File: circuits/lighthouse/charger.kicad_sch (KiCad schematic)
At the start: 15 parts, among them Q2 FS8205A, U4 TP4056-42-ESOP8, U5 DW01A

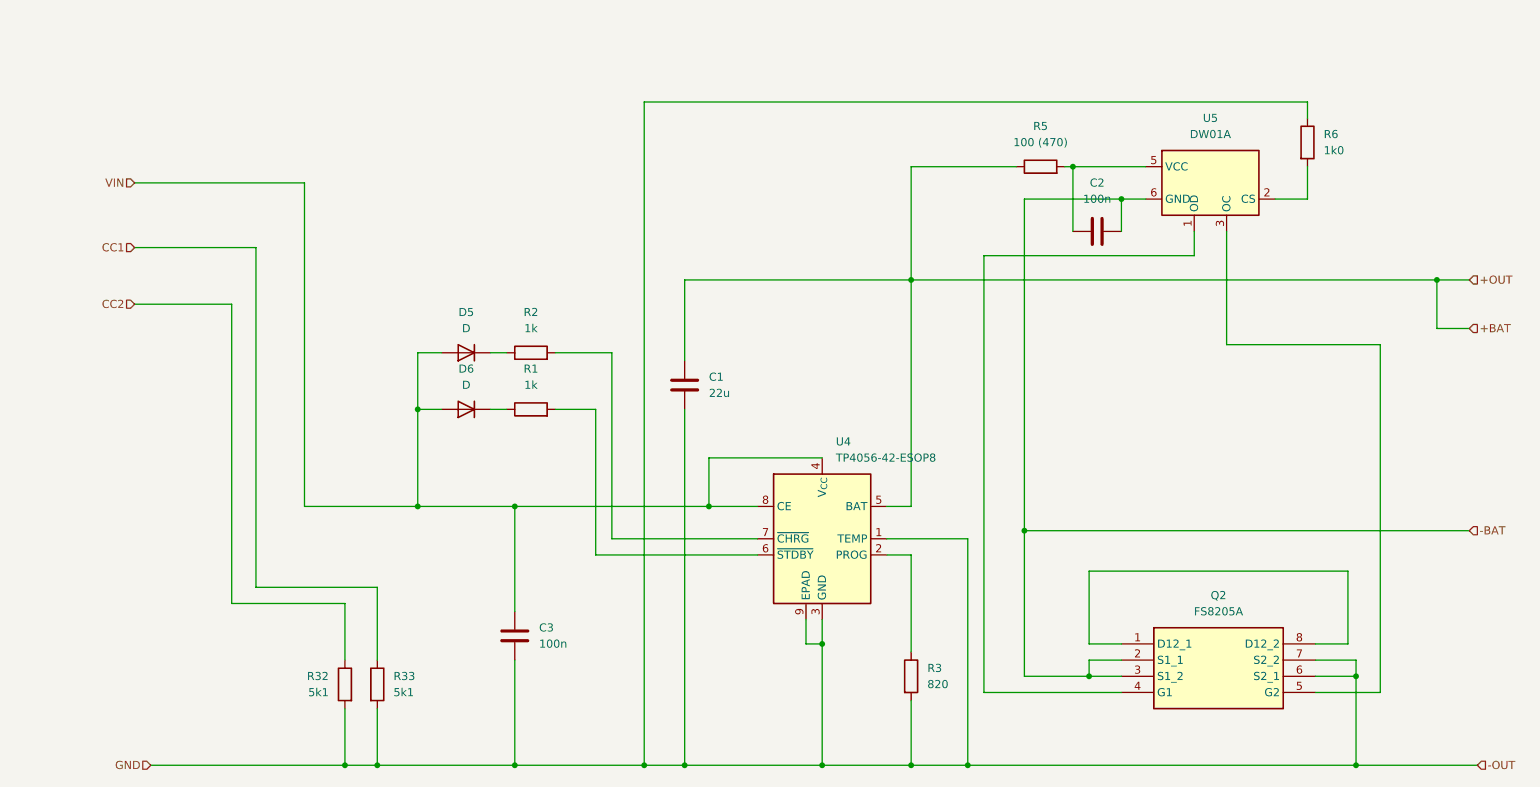
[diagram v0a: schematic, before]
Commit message: Cleaned up schematics
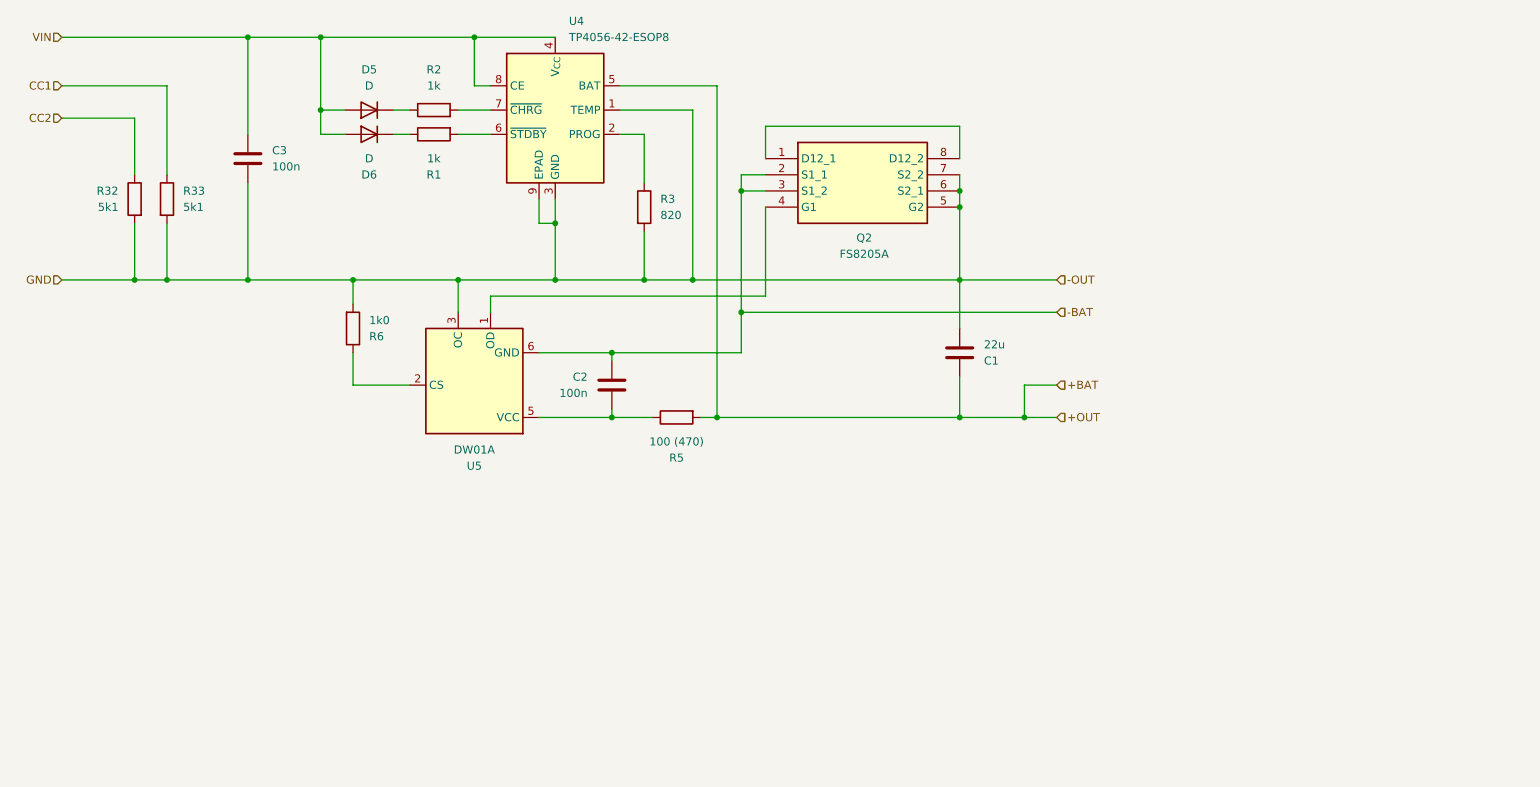
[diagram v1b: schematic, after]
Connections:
- net +BAT: now also R5.2; no longer R5.1
- net -OUT: now also Q2.5 (G2), R6.2, U5.3 (OC); no longer R6.1
- net at C2.1, U5.5 (VCC): now also R5.1; no longer R5.2
- net at U5.2 (CS): now also R6.1; no longer R6.2
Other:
- moved on the sheet: C1, C2, C3, D5, D6, Q2, R1, R2, R3, R32, R33, R5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

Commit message: Sorted out pcb layers
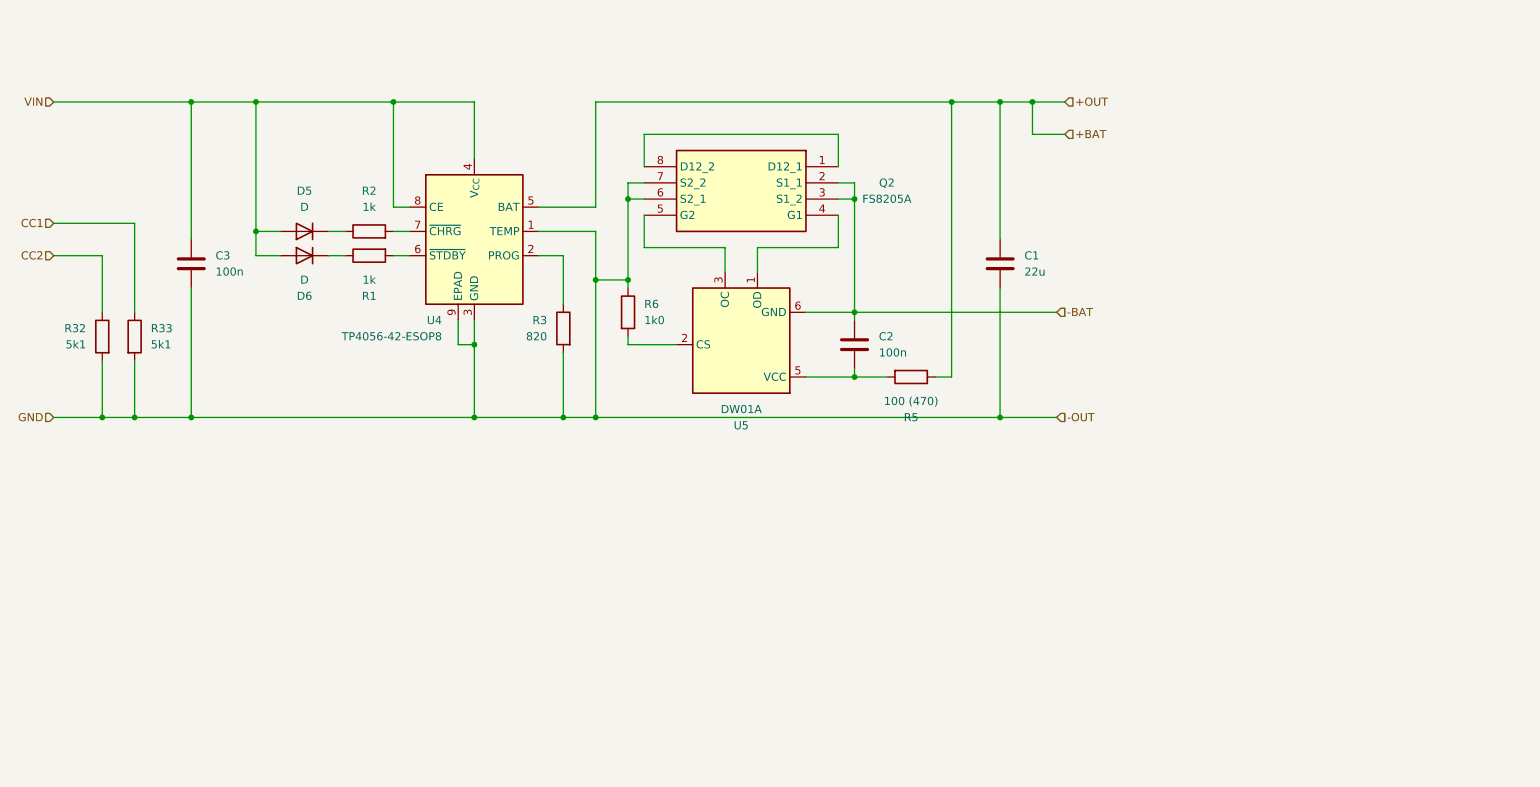
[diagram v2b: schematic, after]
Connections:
- net +BAT: now also R5.1; no longer R5.2
- net -OUT: now also R6.1; no longer Q2.5 (G2), R6.2, U5.3 (OC)
- net at C2.1, U5.5 (VCC): now also R5.2; no longer R5.1
- net at U5.2 (CS): now also R6.2; no longer R6.1
- new net: Q2.5 (G2), U5.3 (OC)
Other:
- moved on the sheet: C1, C2, C3, D5, D6, Q2, R1, R2, R3, R32, R33, R5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
